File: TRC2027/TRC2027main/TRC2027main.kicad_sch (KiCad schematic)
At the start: 68 parts, among them IC1 MCP23017-E_SP, J1 Power_conn(XT90), J10 Memory, J11 BNO055, J12 Temperature, pressure, and al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, J13 Conn_01x03_Pin, J14 Conn_01x04_Pin, J15 Conn_01x04_Pin, J16 Conn_01x04_Pin, J17 Conn_01x04_Pin, J18 Conn_01x04_Pin, J19 Conn_01x12_Pin, J2 電圧計_測定, J20 Conn_01x10_Pin, J21 Conn_01x04_Pin, J22 XH_Moter_Output, J23 XH_Moter_Output, J24 Conn_01x04_Pin, J25 Conn_01x04_Pin, J3 電圧計_電源, J4 XH_Moter_Output, J5 XH_Moter_Output, J6 Conn_01x07_Pin, J7 GPS, J8 Conn_01x08_Pin, J9 Conn_01x08_Pin, SW1 SW_SPST, U1 DCDC, U2 DRV8262DDWR, U3 DRV8262DDWR, U4 DRV8262DDWR, U5 DRV8262DDWR

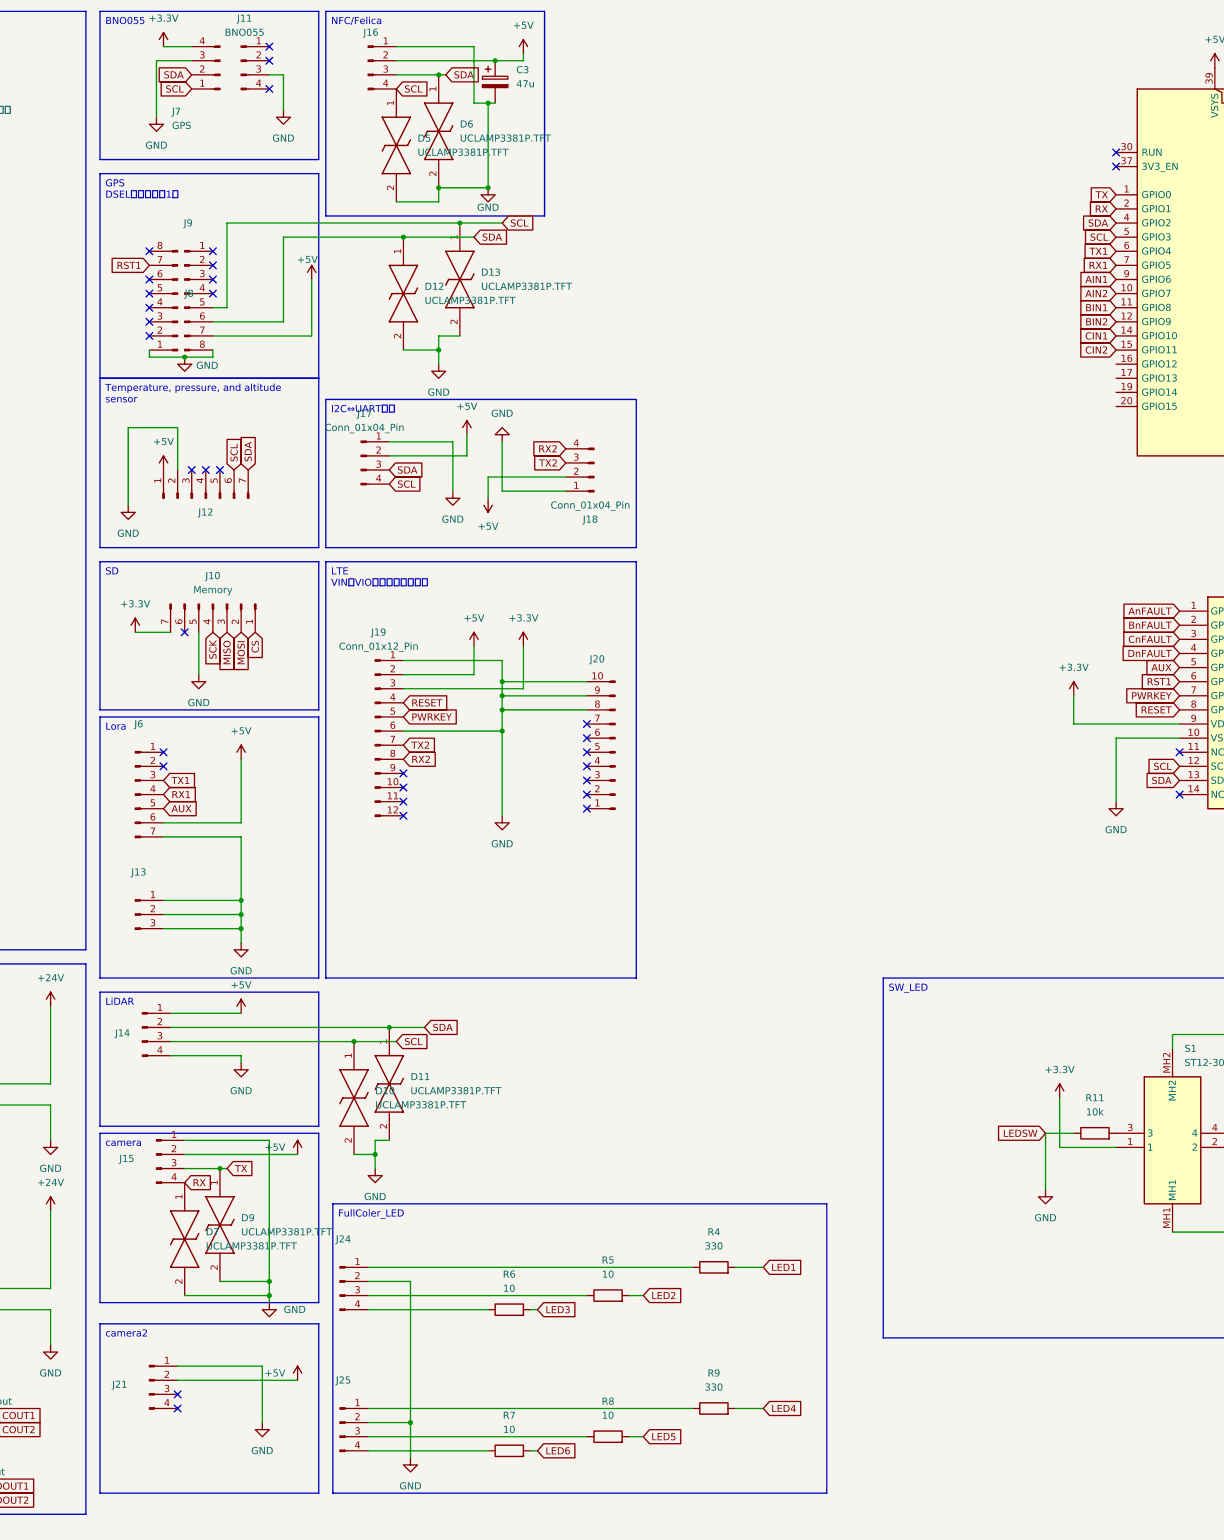
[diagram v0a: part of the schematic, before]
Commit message: new file:   TRC2027/R_Sokutei/R_Sokutei-backups/R_Sokutei-2026-04-18_181141.zip
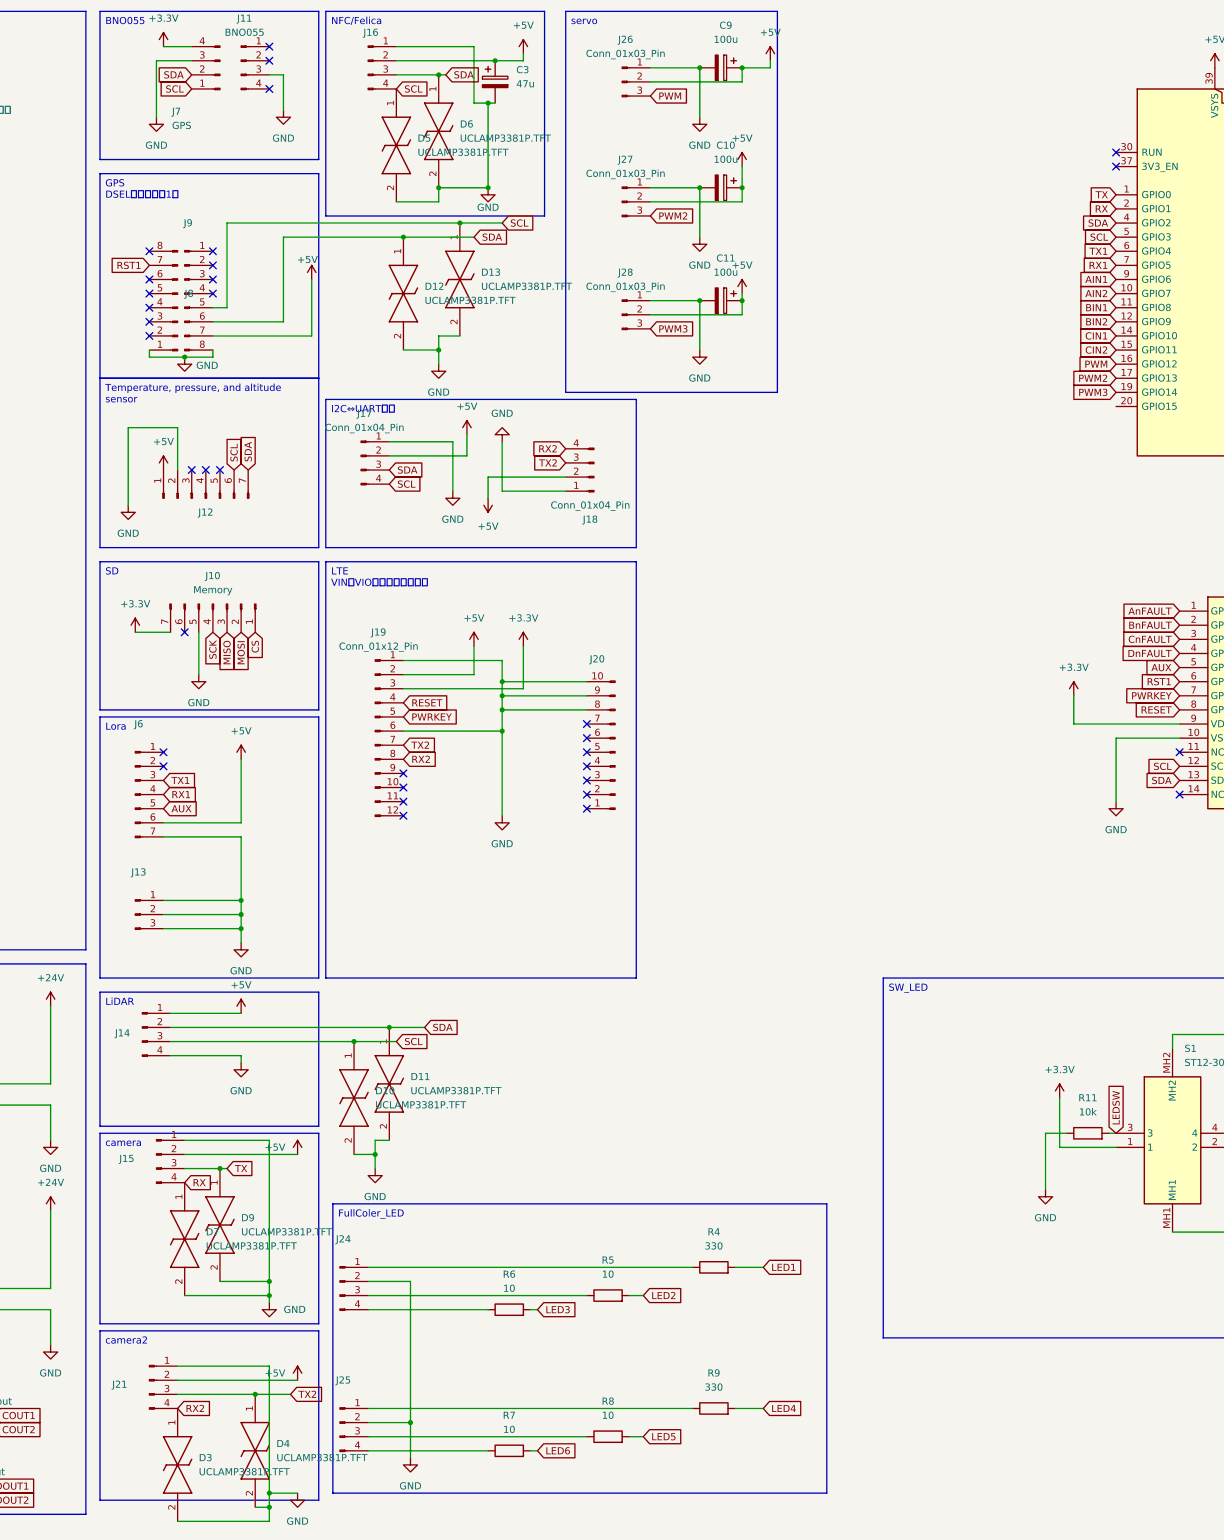
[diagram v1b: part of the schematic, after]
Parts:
- added C10, C11, C9: 100u, Capacitor_THT:CP_Radial_D8.0mm_P3.50mm, symbol Device:C_Polarized
- added D3, D4: UCLAMP3381P.TFT, KiCad_UCLAMP3381:UCLAMP3381PTFT, symbol UCLAMP3381P_TFT:UCLAMP3381P.TFT
- added J26, J27, J28: Conn_01x03_Pin, Connector_JST:JST_XH_B3B-XH-A_1x03_P2.50mm_Vertical, symbol Connector:Conn_01x03_Pin
- J24, J25: footprint LED_THT:LED_D5.0mm-4_RGB -> Connector_JST:JST_XH_B4B-XH-A_1x04_P2.50mm_Vertical
- MD1: footprint OKL_T_6_W12N_C:MURATA_OKL-T-6-W12N-C_0 -> OKL_T_6_W12N_C:OKL-T&slash_6-W12N-C-Kai
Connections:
- net +5V: now also C10.1, C11.1, C9.1, J26.2 (Pin_2), J27.2 (Pin_2), J28.2 (Pin_2)
- net GND: now also C10.2, C11.2, C9.2, D3.2, D4.2, J26.1 (Pin_1), J27.1 (Pin_1), J28.1 (Pin_1); no longer IC1.27 (GPA6)
- net RX2: now also J21.4 (Pin_4), D3.1
- net TX2: now also J21.3 (Pin_3), D4.1
- net LEDSW: now reaches R11.2, S1.3
- net LEDSW: now also IC1.27 (GPA6)
- net PWM: now reaches A1.16 (GPIO12)
- net PWM: now also J26.3 (Pin_3)
- net PWM2: now reaches A1.17 (GPIO13)
- net PWM2: now also J27.3 (Pin_3)
- net PWM3: now reaches A1.19 (GPIO14)
- net PWM3: now also J28.3 (Pin_3)
- no-connect marks 53 -> 51
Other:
- moved on the sheet: R11

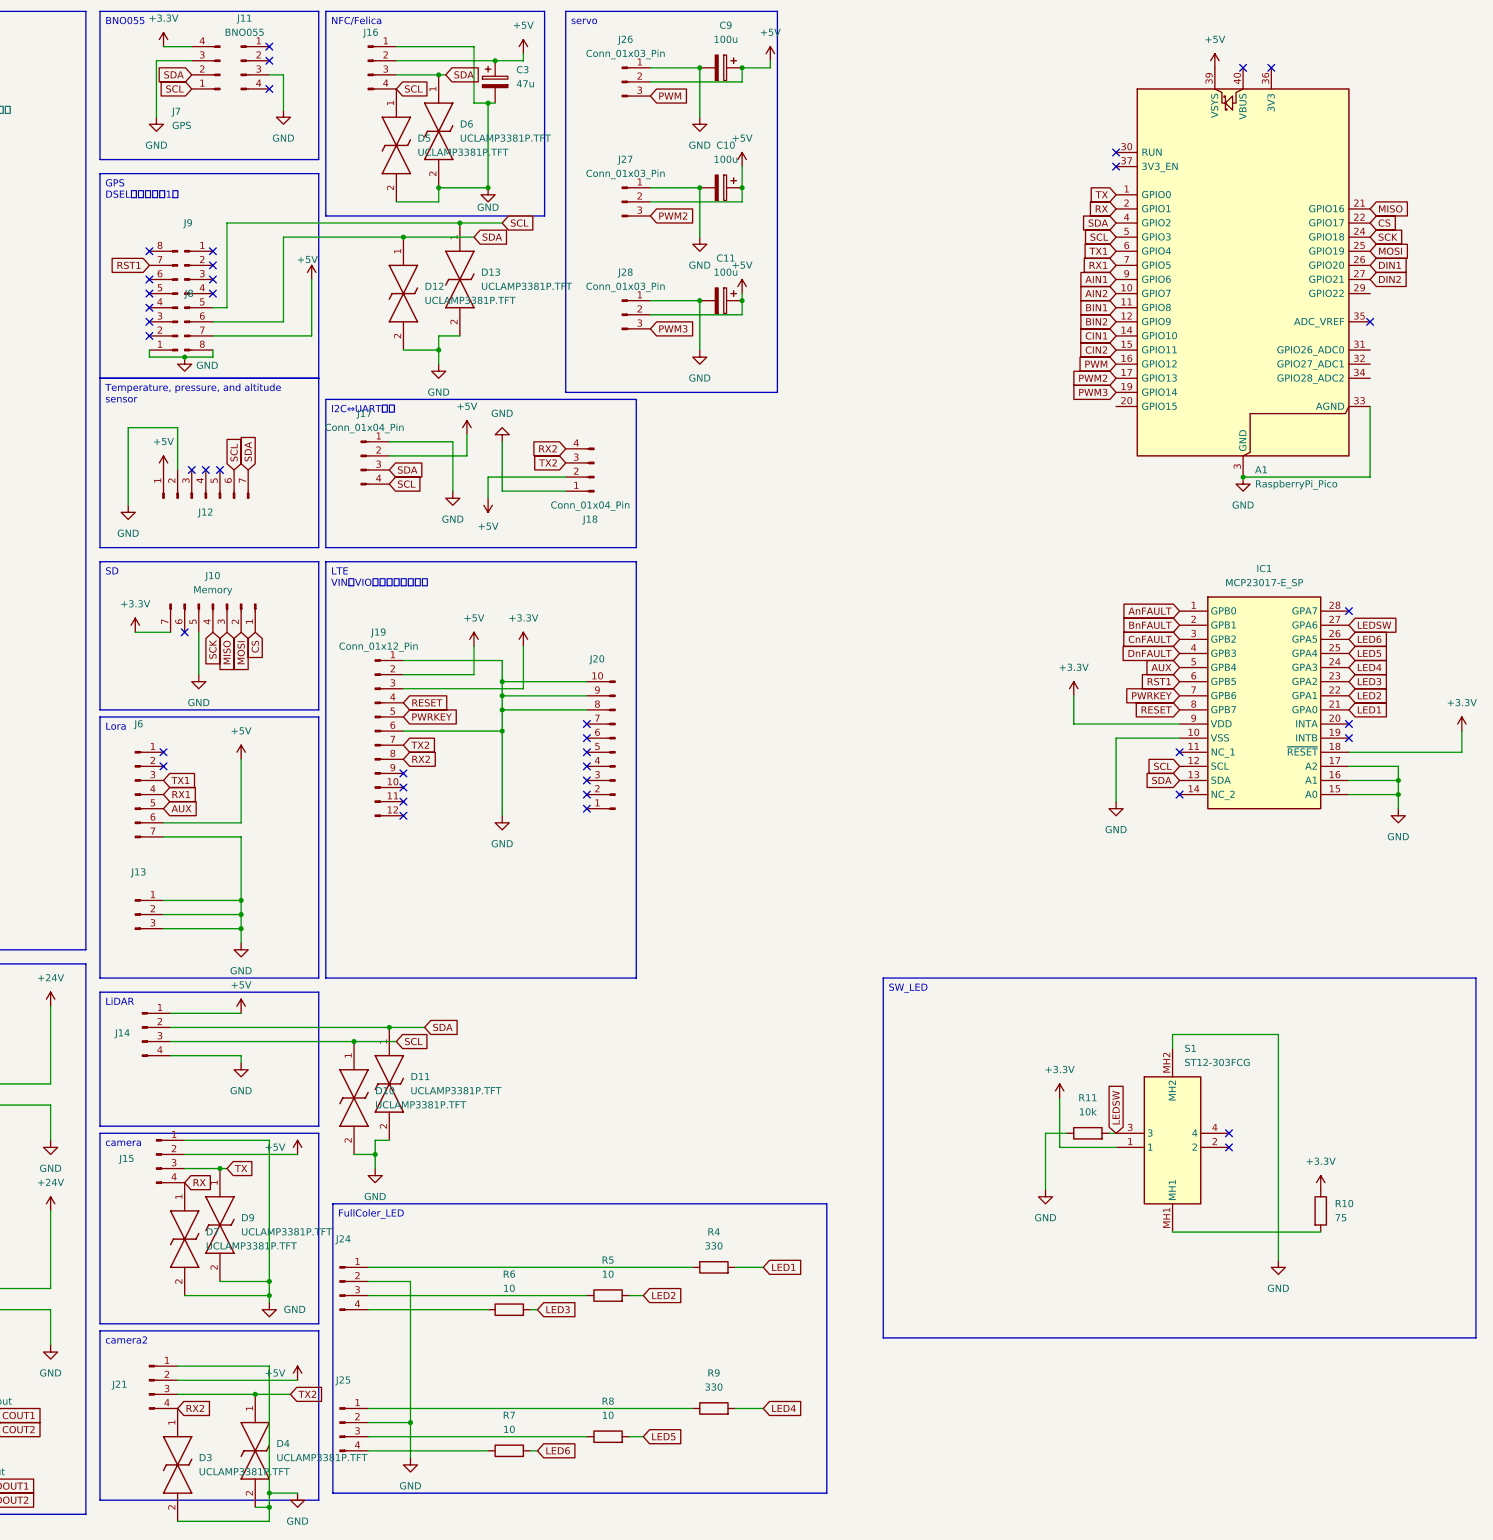
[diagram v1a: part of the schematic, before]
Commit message: add
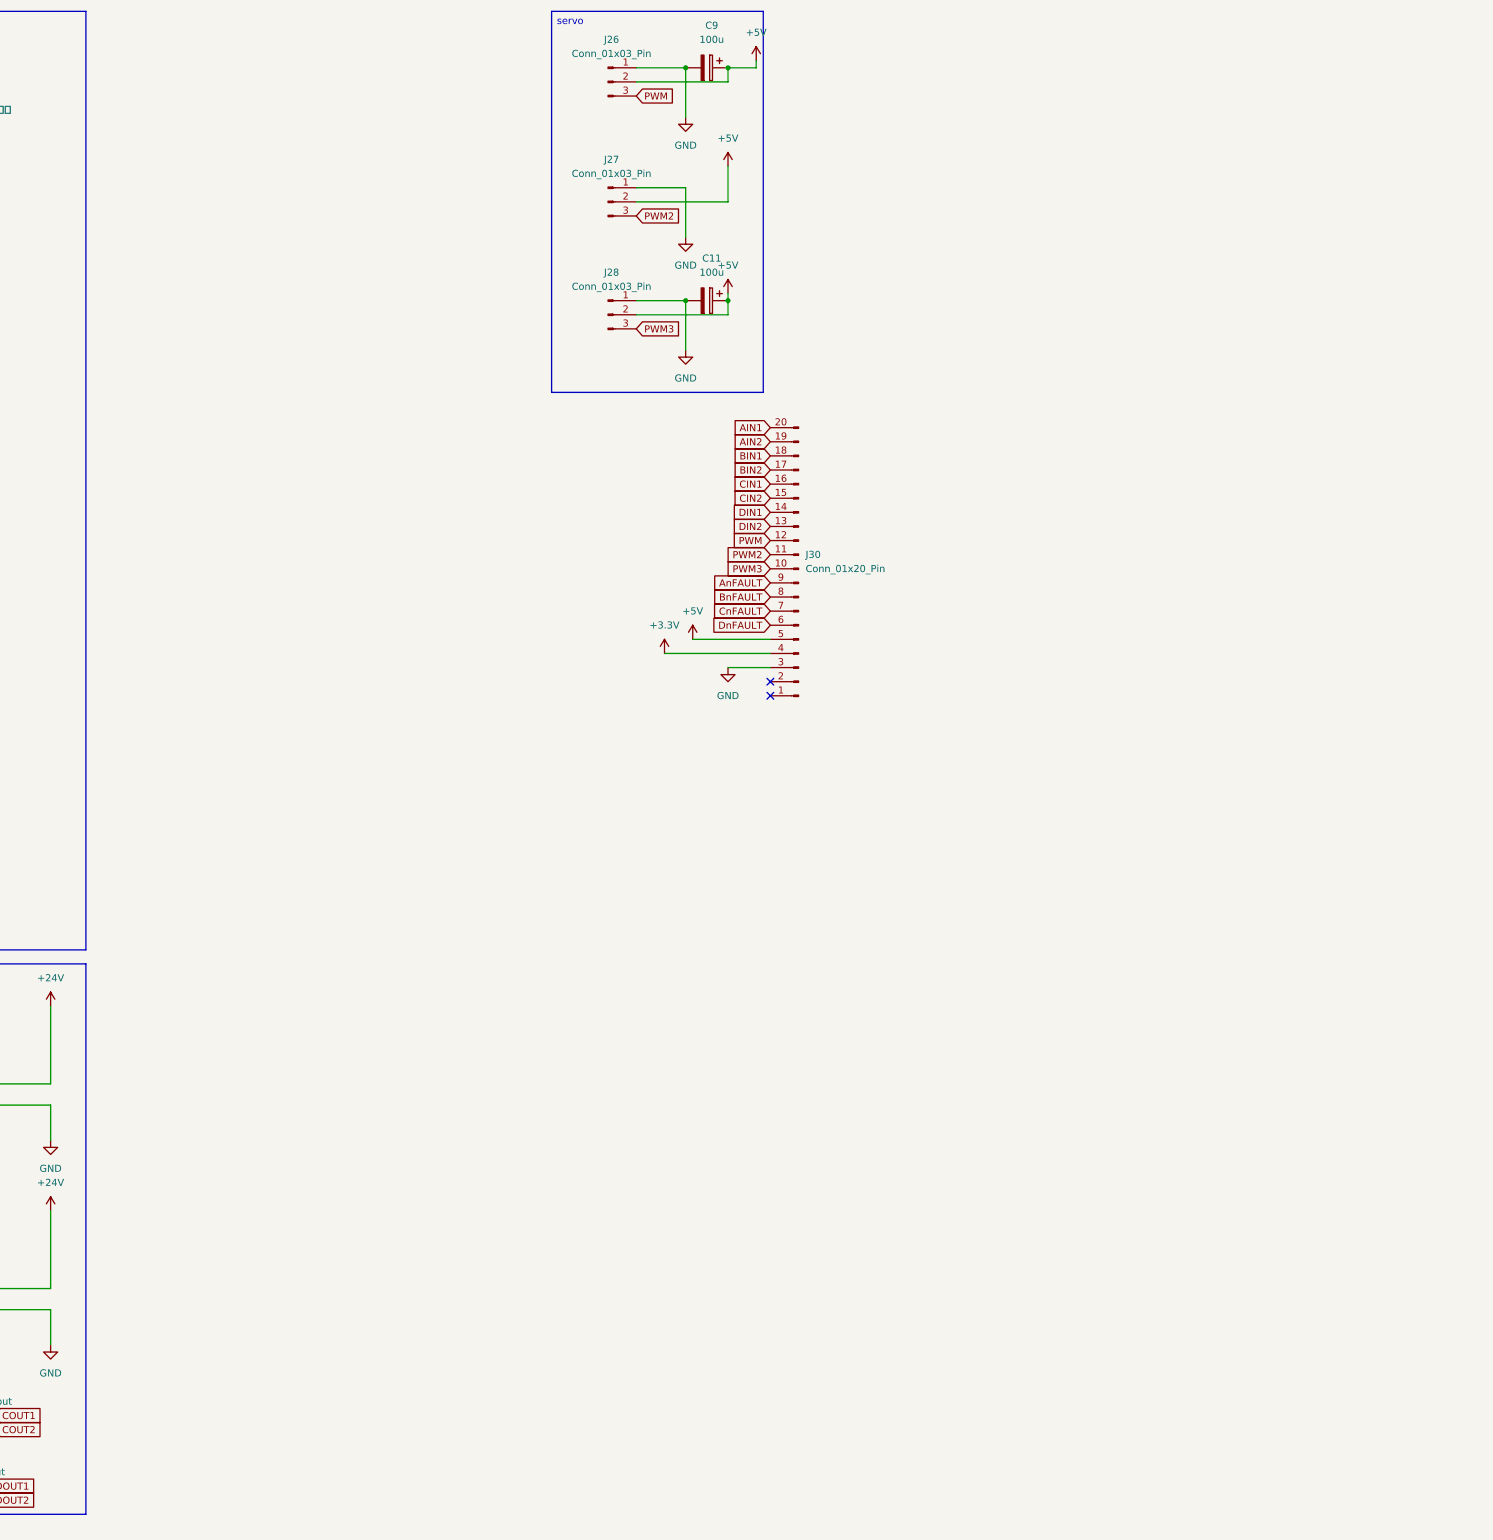
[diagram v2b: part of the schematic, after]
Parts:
- removed A1: RaspberryPi_Pico, Module:RaspberryPi_Pico_Common_Unspecified, symbol MCU_Module:RaspberryPi_Pico
- removed C10: 100u, Capacitor_THT:CP_Radial_D8.0mm_P3.50mm, symbol Device:C_Polarized
- removed C3: 47u, Capacitor_THT:CP_Radial_D5.0mm_P2.00mm, symbol Device:C_Polarized
- removed D10, D11, D12, D13, D3, D4, D5, D6, D7, D9: UCLAMP3381P.TFT, KiCad_UCLAMP3381:UCLAMP3381PTFT, symbol UCLAMP3381P_TFT:UCLAMP3381P.TFT
- removed IC1: MCP23017-E_SP, KiCad_MCP23017:DIP794W56P254L3486H508Q28N, symbol MCP23017-E_SP:MCP23017-E_SP
- removed J10: Memory, Connector_PinSocket_2.54mm:PinSocket_1x07_P2.54mm_Vertical, symbol Connector:Conn_01x07_Pin
- removed J11: BNO055, Connector_PinSocket_2.54mm:PinSocket_1x04_P2.54mm_Vertical, symbol Connector:Conn_01x04_Pin
- removed J12: Temperature, pressure, and altitude sensor, Connector_PinSocket_2.54mm:PinSocket_1x07_P2.54mm_Vertical, symbol Connector:Conn_01x07_Pin
- removed J13: Conn_01x03_Pin, Connector_PinHeader_2.54mm:PinHeader_1x03_P2.54mm_Vertical, symbol Connector:Conn_01x03_Pin
- removed J14, J15, J17, J18, J21, J24, J25: Conn_01x04_Pin, Connector_JST:JST_XH_B4B-XH-A_1x04_P2.50mm_Vertical, symbol Connector:Conn_01x04_Pin
- removed J16: Conn_01x04_Pin, Connector_PinHeader_2.54mm:PinHeader_1x04_P2.54mm_Vertical, symbol Connector:Conn_01x04_Pin
- removed J19: Conn_01x12_Pin, Connector_PinHeader_2.54mm:PinHeader_1x12_P2.54mm_Vertical, symbol Connector:Conn_01x12_Pin
- removed J20: Conn_01x10_Pin, Connector_PinHeader_2.54mm:PinHeader_1x10_P2.54mm_Vertical, symbol Connector:Conn_01x10_Pin
- removed J6: Conn_01x07_Pin, Connector_PinHeader_2.54mm:PinHeader_1x07_P2.54mm_Vertical, symbol Connector:Conn_01x07_Pin
- removed J7: GPS, Connector_PinSocket_2.54mm:PinSocket_1x04_P2.54mm_Vertical, symbol Connector:Conn_01x04_Pin
- removed J8, J9: Conn_01x08_Pin, Connector_PinHeader_2.54mm:PinHeader_1x08_P2.54mm_Vertical, symbol Connector:Conn_01x08_Pin
- removed R10: 75, Resistor_THT:R_Axial_DIN0207_L6.3mm_D2.5mm_P10.16mm_Horizontal, symbol Device:R
- removed R11: 10k, Resistor_THT:R_Axial_DIN0207_L6.3mm_D2.5mm_P10.16mm_Horizontal, symbol Device:R
- removed R4, R9: 330, Resistor_THT:R_Axial_DIN0207_L6.3mm_D2.5mm_P10.16mm_Horizontal, symbol Device:R
- removed R5, R6, R7, R8: 10, Resistor_THT:R_Axial_DIN0207_L6.3mm_D2.5mm_P10.16mm_Horizontal, symbol Device:R
- removed S1: ST12-303FCG, KiCad_ST12:ST12303FCG, symbol ST12-303FCG:ST12-303FCG
- added J30: Conn_01x20_Pin, Connector_JST:JST_XH_B20B-XH-A_1x20_P2.50mm_Vertical, symbol Connector:Conn_01x20_Pin
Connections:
- net +3.3V: now also J30.4 (Pin_4)
- net +5V: now also J30.5 (Pin_5)
- net AIN1: now also J30.20 (Pin_20)
- net AIN2: now also J30.19 (Pin_19)
- net AnFAULT: now also J30.9 (Pin_9)
- net BIN1: now also J30.18 (Pin_18)
- net BIN2: now also J30.17 (Pin_17)
- net BnFAULT: now also J30.8 (Pin_8)
- net CIN1: now also J30.16 (Pin_16)
- net CIN2: now also J30.15 (Pin_15)
- net CnFAULT: now also J30.7 (Pin_7)
- net DIN1: now also J30.14 (Pin_14)
- net DIN2: now also J30.13 (Pin_13)
- net DnFAULT: now also J30.6 (Pin_6)
- net GND: now also J30.3 (Pin_3)
- net PWM: now also J30.12 (Pin_12)
- net PWM2: now also J30.11 (Pin_11)
- net PWM3: now also J30.10 (Pin_10)
- no-connect marks 51 -> 11
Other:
- moved on the sheet: C11, C9, J26, J27, J28
